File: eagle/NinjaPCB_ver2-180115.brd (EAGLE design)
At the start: 73 x 73 mm, 55 parts, among them IC3 ANALOGSW_AD_SOT23-6NC, IC4 ANALOGSW_TI-SC70-5/6NC, IC6 NAU7802NC, J1 PELTIER, J2 ATX24, J3 HEATER, J4 HEATER_TEMP, Q1 S9013, Q2 IRF520NPBF, Q3 IRF520NPBF, Q4 S9013, Q5 IRF520NPBF, Q6 S9013, Q7 S9013, Q8 S9013, U1 CJT1117-3.3-SOT223

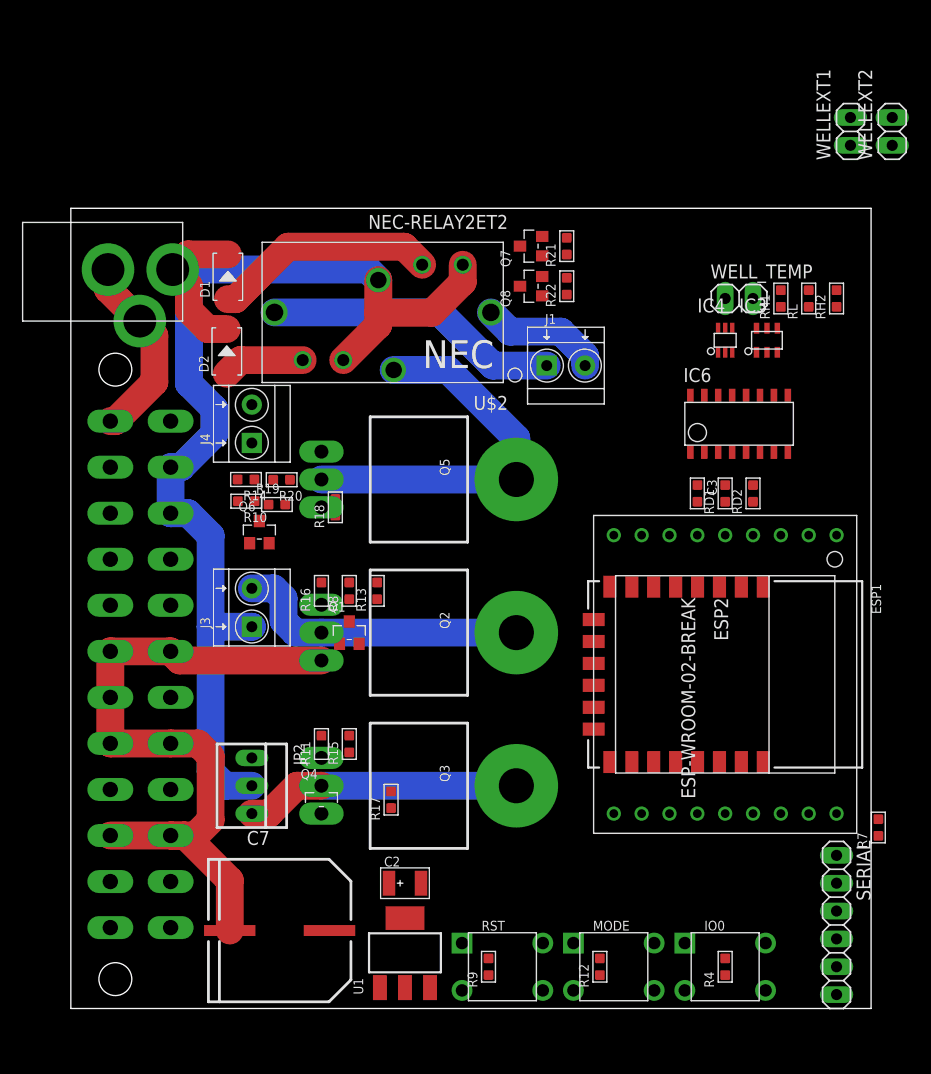
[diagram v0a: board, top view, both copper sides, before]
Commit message: finished
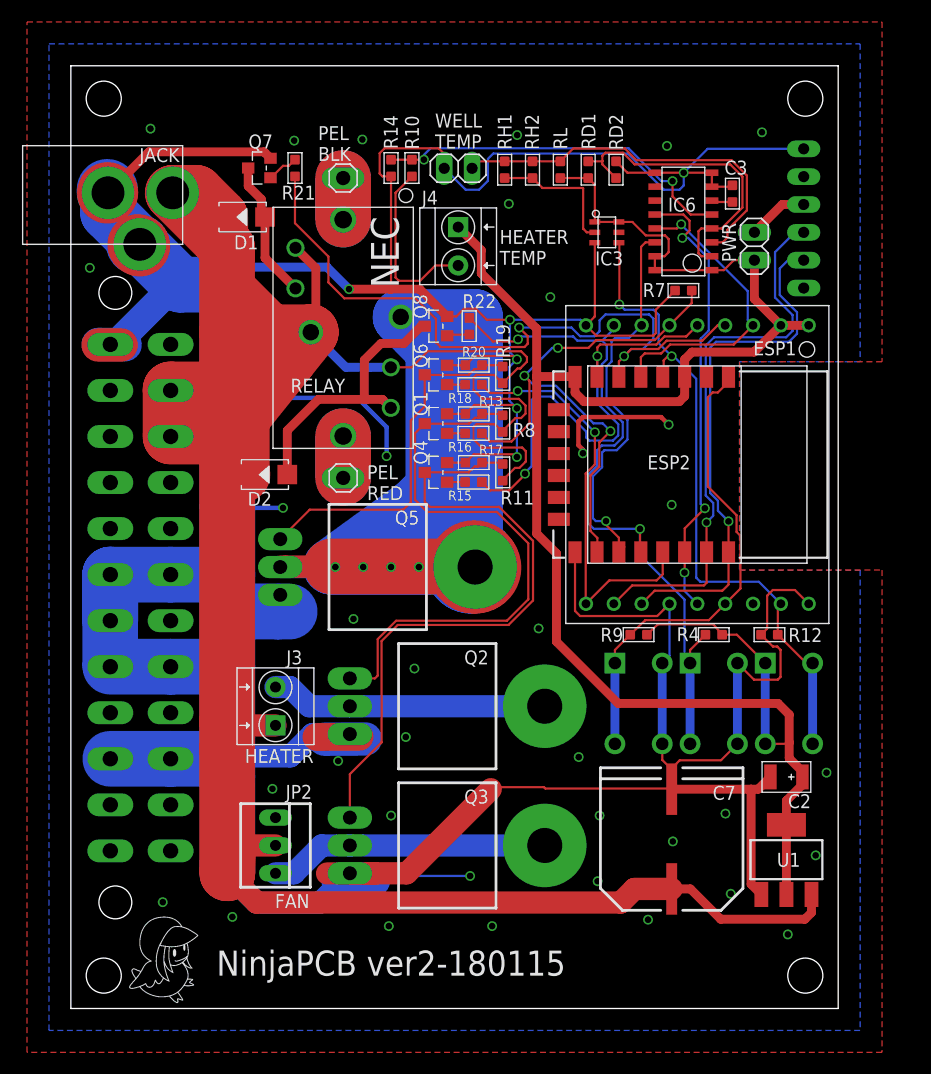
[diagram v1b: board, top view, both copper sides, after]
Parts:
- removed IC4: ANALOGSW_TI-SC70-5/6NC, PCR-IC:SC70-6NC
- removed J1: PELTIER, Seeed-Connector:H2-3.5-7.0X7.0MM
- removed WELLEXT1, WELLEXT2: (no value), pinhead:1X02
- added JACK: 2.1MMJACKTHM, adafruit:PJ-102A
- added PEL_BLK, PEL_RED: (no value), pinhead:1X01LONG
- added PWR: (no value), pinhead:1X02
- added RELAY: NEC-RELAY2ET2, PCR-Switch:NEC-ET2-N8
- IC3: value ANALOGSW_AD_SOT23-6NC -> ANALOGSW_AD_SOT23-6; device PCR-IC:SOT-23-6NC -> PCR-IC:SOT-23-6
- IC6: value NAU7802NC -> NAU7802; device PCR-IC:SOP-16NC -> PCR-IC:SOP-16
- RD1, RD2, RH1, RH2, RL: device PCR-RCL:R0603NC -> PCR-RCL:R0603
- U$1: value 2.1MMJACKTHM -> (none); device adafruit:PJ-102A -> PCR-Logo:TORI_0.25
- U$2: value NEC-RELAY2ET2 -> (none); device PCR-Switch:NEC-ET2-N8 -> PCR-Logo:TORI_0.25
- moved U$2 73.0 mm to (65.3, 0.43), flipped to the bottom, turned to 0 degrees
- moved U$1 67.1 mm to (5.18, 0.38), turned to 0 degrees
- moved SERIAL 64.5 mm to (66.9, 72.1), flipped to the bottom, turned to 90 degrees
- moved R7 52.1 mm to (55.9, 65.5), turned to 90 degrees
- moved C7 36.7 mm to (54.8, 15.5), turned to 180 degrees
- moved C2 36.1 mm to (65.3, 21.1), turned to 180 degrees
- moved U1 35.8 mm to (65.3, 13.6)
- moved R12 34.0 mm to (63.7, 34.1), turned to 90 degrees
- moved R10 33.9 mm to (31.1, 76.7), turned to 0 degrees
- moved R9 33.2 mm to (51.8, 34.1), turned to 270 degrees
- moved RD1 32.1 mm to (47.2, 76.5)
- moved RD2 32.1 mm to (49.7, 76.5)
- moved R17 31.7 mm to (36.8, 49.8), turned to 90 degrees
- moved Q4 31.6 mm to (33.3, 48.9), turned to 90 degrees
- moved R14 31.3 mm to (29.2, 76.7), turned to 0 degrees
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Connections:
- removed net N$26: WELLEXT1.1, WELLEXT2.1
- removed net N$28: WELLEXT1.2, WELLEXT2.2
- removed net PEL_INA: ESP1.6, ESP2.P$4
- removed net PEL_INB: ESP1.18, ESP2.P$8, IO0.1, IO0.4, R4.2
- new net PWR: PWR.1, SERIAL.4
- net 12V: now also JACK.TIP, RELAY.P$2, RELAY.P$4, RELAY.P$6; no longer U$1.TIP, U$2.P$2, U$2.P$4, U$2.P$6
- net 3V3: now also J4.1, PWR.2; no longer IC4.P$1, IC4.P$6, J4.2
- net GND: now also JACK.RING, JACK.RING_SW; no longer IC4.P$3, U$1.RING, U$1.RING_SW
- net HIGH_TEMP: no longer IC4.P$4
- net N$1: now also J4.2; no longer J4.1
- net N$27: no longer IC4.P$2
- net N$3: now also RELAY.P$5; no longer U$2.P$5
- net N$33: now also RELAY.P$3; no longer U$2.P$3
- net N$36: now also RELAY.P$7; no longer U$2.P$7
- net N$6: now also PEL_RED.1, RELAY.P$8; no longer J1.1, U$2.P$8
- net N$7: now also PEL_BLK.1, RELAY.P$1; no longer J1.2, U$2.P$1
- net PEL_SWA: now also ESP1.6, ESP2.P$4
- net PEL_SWB: now also ESP1.18, ESP2.P$8, IO0.1, IO0.4, R4.2
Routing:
- net GND: track 82.4 -> 528.5 mm, vias 0 -> 42
- net 3V3: track 0.00 -> 171.4 mm
- net 12V: track 112.4 -> 258.7 mm
- net N$3: track 36.5 -> 136.7 mm, vias 0 -> 4
- net PEL_SWB: track 0.00 -> 67.4 mm, vias 0 -> 2
- net PEL_SWA: track 0.00 -> 66.5 mm, vias 0 -> 2
- net HIGH_TEMP: track 0.00 -> 60.8 mm, vias 0 -> 2
- net N$25: track 0.00 -> 59.7 mm
- net N$29: track 0.00 -> 53.2 mm
- net RXD: track 0.00 -> 51.1 mm, vias 0 -> 1
- net HEATER: track 0.00 -> 51.1 mm, vias 0 -> 3
- net TXD: track 0.00 -> 48.5 mm, vias 0 -> 1
- net RESET: track 0.00 -> 43.9 mm
- net FAN: track 0.00 -> 42.8 mm, vias 0 -> 2
- net DRDY: track 0.00 -> 41.6 mm, vias 0 -> 3
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- added copper zone on layer 1, net GND
- added copper zone on layer 16, net GND
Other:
- board size 73 x 73 mm -> 70 x 86 mm
- board text added: "FAN"
- board text added: "GND"
- board text added: "HEATER"
- board text added: "HEATER TEMP"
- board text added: "JACK"
- board text added: "NinjaPCB ver2-180115"
- board text added: "PEL BLK"
- board text added: "PEL RED"
- board text added: "PWR"
- board text added: "RELAY"
- board text added: "RX"
- board text added: "TX"
- board text added: "WELL TEMP"
